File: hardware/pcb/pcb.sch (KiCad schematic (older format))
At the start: 15 parts, among them Q1 FDN339AN, SW1 SW_SPST, U1 WeMos_D1_mini, U2 TSOP38236

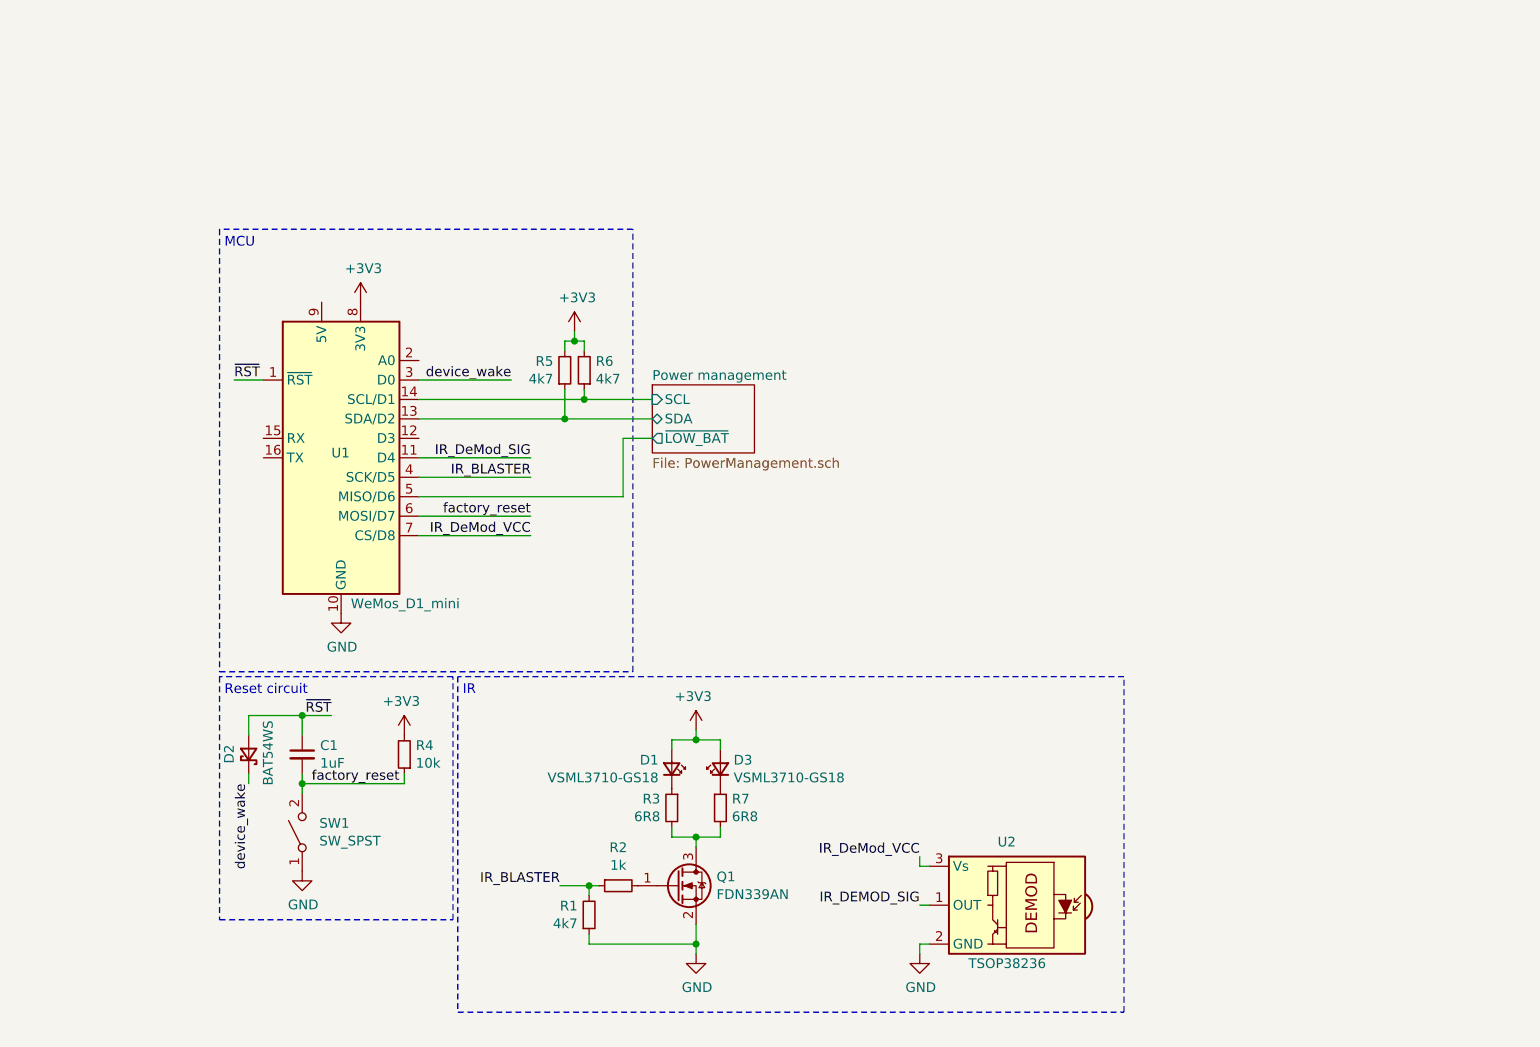
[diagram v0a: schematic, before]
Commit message: Added schematic
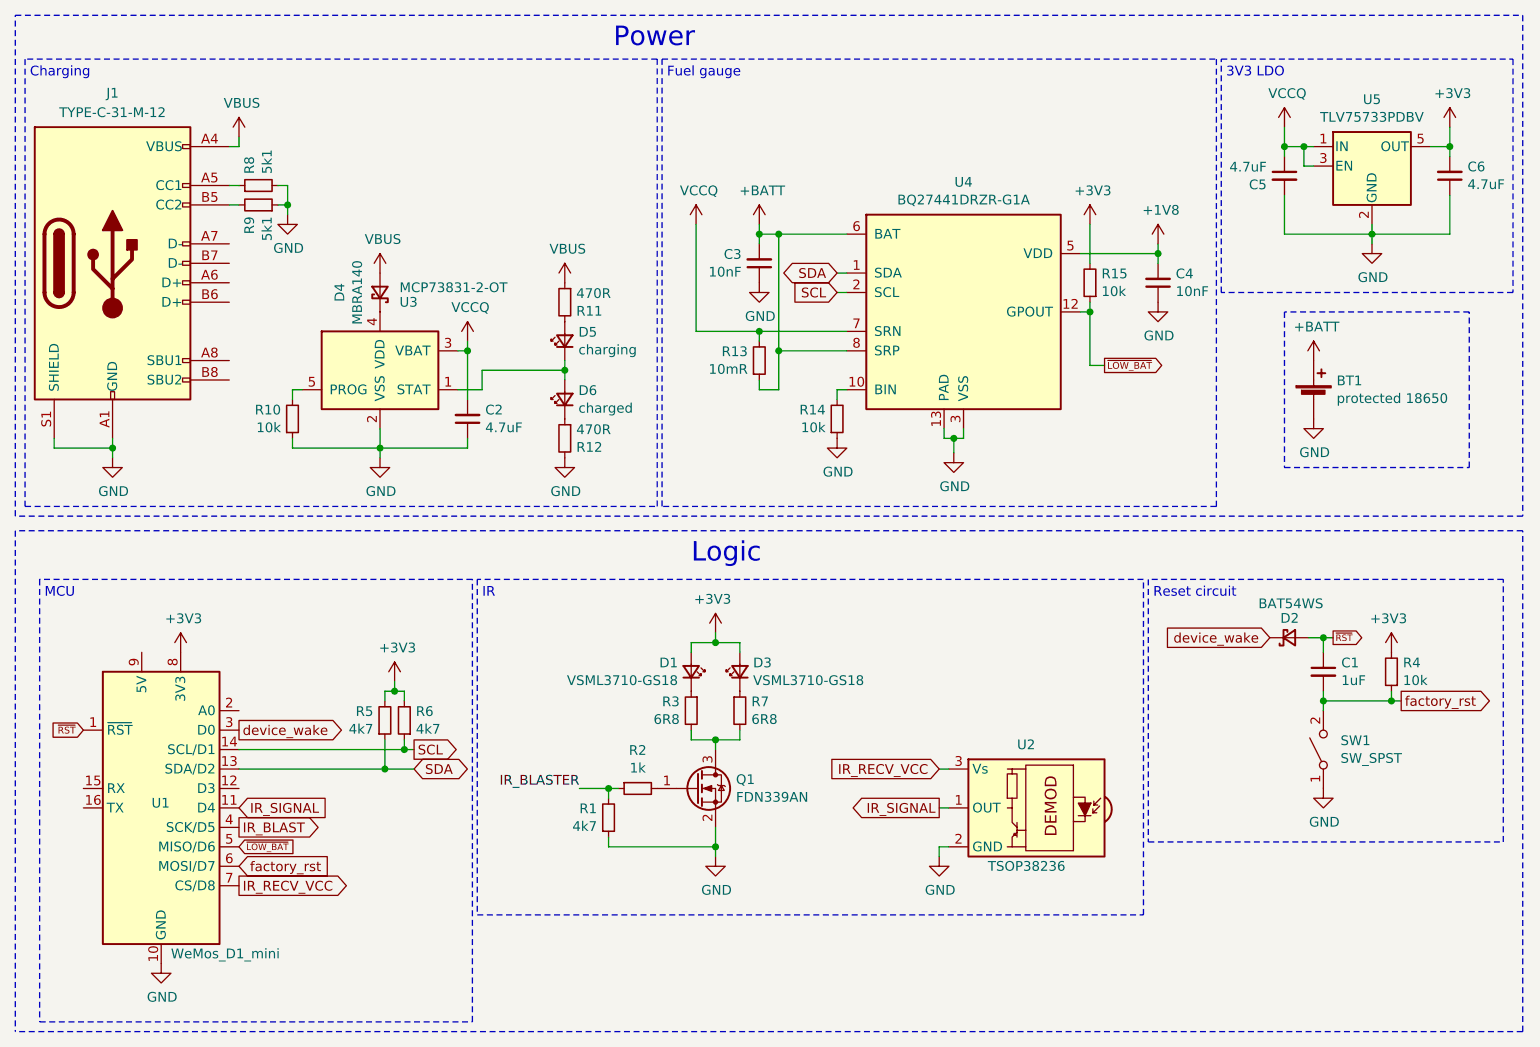
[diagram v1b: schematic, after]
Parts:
- added BT1: protected 18650, Battery:BatteryHolder_Keystone_1042_1x18650, symbol Device:Battery_Cell
- added C2, C5, C6: 4.7uF, Capacitor_SMD:C_0805_2012Metric_Pad1.15x1.40mm_HandSolder, symbol Device:C_Small
- added C3, C4: 10nF, Capacitor_SMD:C_0603_1608Metric_Pad1.05x0.95mm_HandSolder, symbol Device:C_Small
- added D4: MBRA140, Diode_SMD:D_SMA, symbol Device:D_Schottky_Small
- added D5: charging, LED_SMD:LED_0603_1608Metric_Pad1.05x0.95mm_HandSolder, symbol Device:LED_Small
- added D6: charged, LED_SMD:LED_0603_1608Metric_Pad1.05x0.95mm_HandSolder, symbol Device:LED_Small
- added J1: TYPE-C-31-M-12, Connector_USB:USB_C_Receptacle_HRO_TYPE-C-31-M-12, symbol Connector:USB_C_Receptacle_USB2.0
- added R10, R14, R15: 10k, Resistor_SMD:R_0603_1608Metric_Pad1.05x0.95mm_HandSolder, symbol Device:R_Small
- added R11, R12: 470R, Resistor_SMD:R_0603_1608Metric_Pad1.05x0.95mm_HandSolder, symbol Device:R_Small
- added R13: 10mR, Resistor_SMD:R_0603_1608Metric_Pad1.05x0.95mm_HandSolder, symbol Device:R_Small
- added R8, R9: 5k1, Resistor_SMD:R_0603_1608Metric_Pad1.05x0.95mm_HandSolder, symbol Device:R_Small
- added U3: MCP73831-2-OT, Package_TO_SOT_SMD:SOT-23-5, symbol Battery_Management:MCP73831-2-OT
- added U4: BQ27441DRZR-G1A, Package_SON:Texas_S-PDSO-N12, symbol Battery_Management:BQ27441DRZR-G1A
- added U5: TLV75733PDBV, Package_TO_SOT_SMD:SOT-23-5, symbol Regulator_Linear:TLV75733PDBV
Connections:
- net IR_DeMod_SIG is gone; now on net IR_SIGNAL: U1.11 (D4)
- net +3V3: now also C6.2, R15.2, U5.5 (OUT)
- net GND: now also BT1.2 (-), C2.1, C3.1, C4.1, C5.2, C6.1, J1.A1 (GND), J1.A12 (GND), J1.B1 (GND), J1.B12 (GND), J1.S1 (SHIELD), R10.1, R12.2, R14.1, R8.2, R9.1, U3.2 (VSS), U4.13 (PAD), U4.3 (VSS), U5.2 (GND)
- net IR_BLASTER: no longer U1.4 (SCK/D5)
- net IR_DEMOD_SIG renamed IR_SIGNAL
- net IR_DeMod_VCC renamed IR_RECV_VCC
- net Power management/SCL renamed SCL
- net SCL: now also U4.2 (SCL)
- net Power management/SDA renamed SDA
- net SDA: now also U4.1 (SDA)
- net Power management/~LOW_BAT renamed ~LOW_BAT
- net ~LOW_BAT: now also R15.1, U4.12 (GPOUT)
- net factory_reset renamed factory_rst
- new net: J1.A5 (CC1), R8.1
- new net: J1.B5 (CC2), R9.2
- new net: R14.2, U4.10 (BIN)
- new net: D5.2 (A), R11.2
- new net: D5.1 (K), D6.2 (A), U3.1 (STAT)
- new net: D6.1 (K), R12.1
- new net: D4.1 (K), U3.4 (VDD)
- new net: R10.2, U3.5 (PROG)
- new net +1V8: C4.2, U4.5 (VDD)
- new net +BATT: BT1.1 (+), C3.2, R13.1, U4.6 (BAT), U4.8 (SRP)
- new net IR_BLAST: U1.4 (SCK/D5)
- new net VBUS: D4.2 (A), J1.A4 (VBUS), J1.A9 (VBUS), J1.B4 (VBUS), J1.B9 (VBUS), R11.1
- new net VCCQ: C2.2, C5.1, R13.2, U3.3 (VBAT), U4.7 (SRN), U5.1 (IN), U5.3 (EN)
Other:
- note added: "3V3 LDO"
- note added: "Charging"
- note added: "Fuel gauge"
- note added: "Logic"
- note added: "Power"
- moved on the sheet: C1, D1, D2, D3, Q1, R1, R2, R3, R4, R5, R6, R7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
